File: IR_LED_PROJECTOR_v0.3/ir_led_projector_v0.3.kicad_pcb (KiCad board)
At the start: 2 copper layers, 42 x 40.3 mm, 31 parts, among them Q1 Q_NMOS_DGS, U1 AZ1084-ADJ

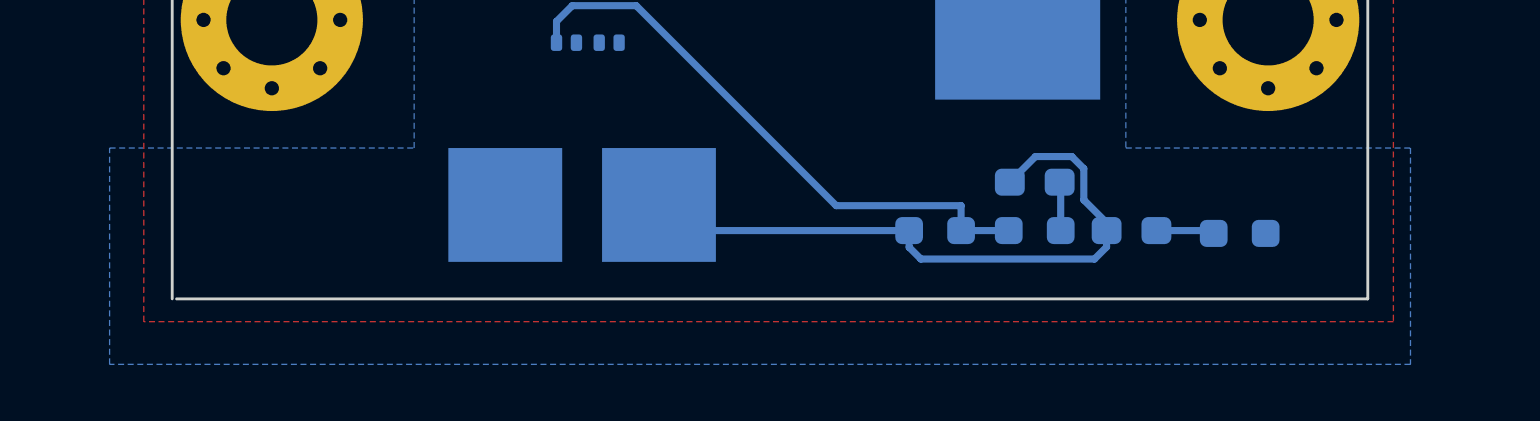
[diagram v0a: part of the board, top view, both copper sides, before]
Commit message: add gripper and so on
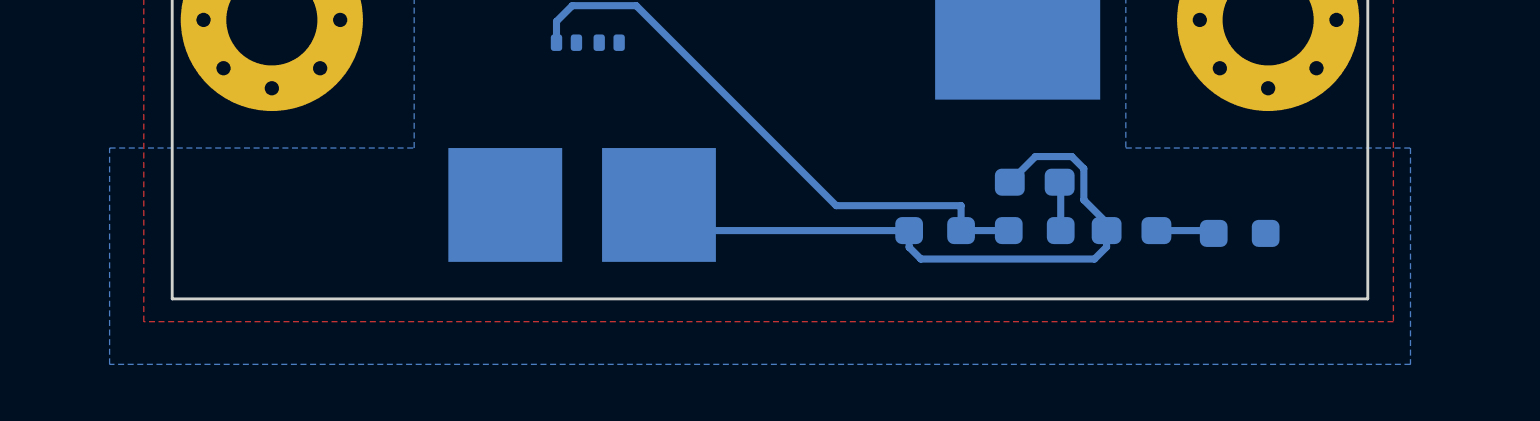
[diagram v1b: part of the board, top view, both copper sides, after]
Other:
- outline, holes or cut-outs redrawn
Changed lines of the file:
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@@
   (gr_line locked (start 100 117.5) (end 135 117.5) (layer "Dwgs.User") (width 0.15))
   (gr_line (start 138.5 140.3) (end 138.5 100) (layer "Edge.Cuts") (width 0.1))
-  (gr_line (start 96.65 140.3) (end 138.5 140.3) (layer "Edge.Cuts") (width 0.1))
+  (gr_line (start 96.5 140.3) (end 138.5 140.3) (layer "Edge.Cuts") (width 0.1))
   (gr_line (start 96.5 100) (end 96.5 140.3) (layer "Edge.Cuts") (width 0.1))
   (gr_line (start 96.5 100) (end 138.5 100) (layer "Edge.Cuts") (width 0.1))
@@
   (zone (net 18) (net_name "/IN") (layers F&B.Cu) (name "VCC") (hatch edge 0.508)
     (priority 5)
-    (connect_pads yes (clearance 0.508))
+    (connect_pads yes (clearance 0.5))
     (min_thickness 0.254) (filled_areas_thickness no)
     (fill yes (thermal_gap 0.508) (thermal_bridge_width 0.508) (smoothing fillet) (radius 1) (island_removal_mode 2) (island_area_min 0))
@@
   (zone (net 19) (net_name "/OUT") (layer "B.Cu") (name "GND") (hatch edge 0.508)
     (priority 5)
-    (connect_pads yes (clearance 0.508))
+    (connect_pads yes (clearance 0.5))
     (min_thickness 0.254) (filled_areas_thickness no)
     (fill yes (thermal_gap 0.508) (thermal_bridge_width 0.508) (island_removal_mode 2) (island_area_min 0))
